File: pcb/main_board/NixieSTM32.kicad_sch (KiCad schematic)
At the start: 36 parts, among them J1 Conn_ARM_SWD_6, Q1 FQU11P06TU, SW1 SW_SPDT, U1 STM32L010K4T6, U2 MAX6817, U3 TPS7A05SOT23, U4 LT3470ITS8PBF, Y1 32.768kHz

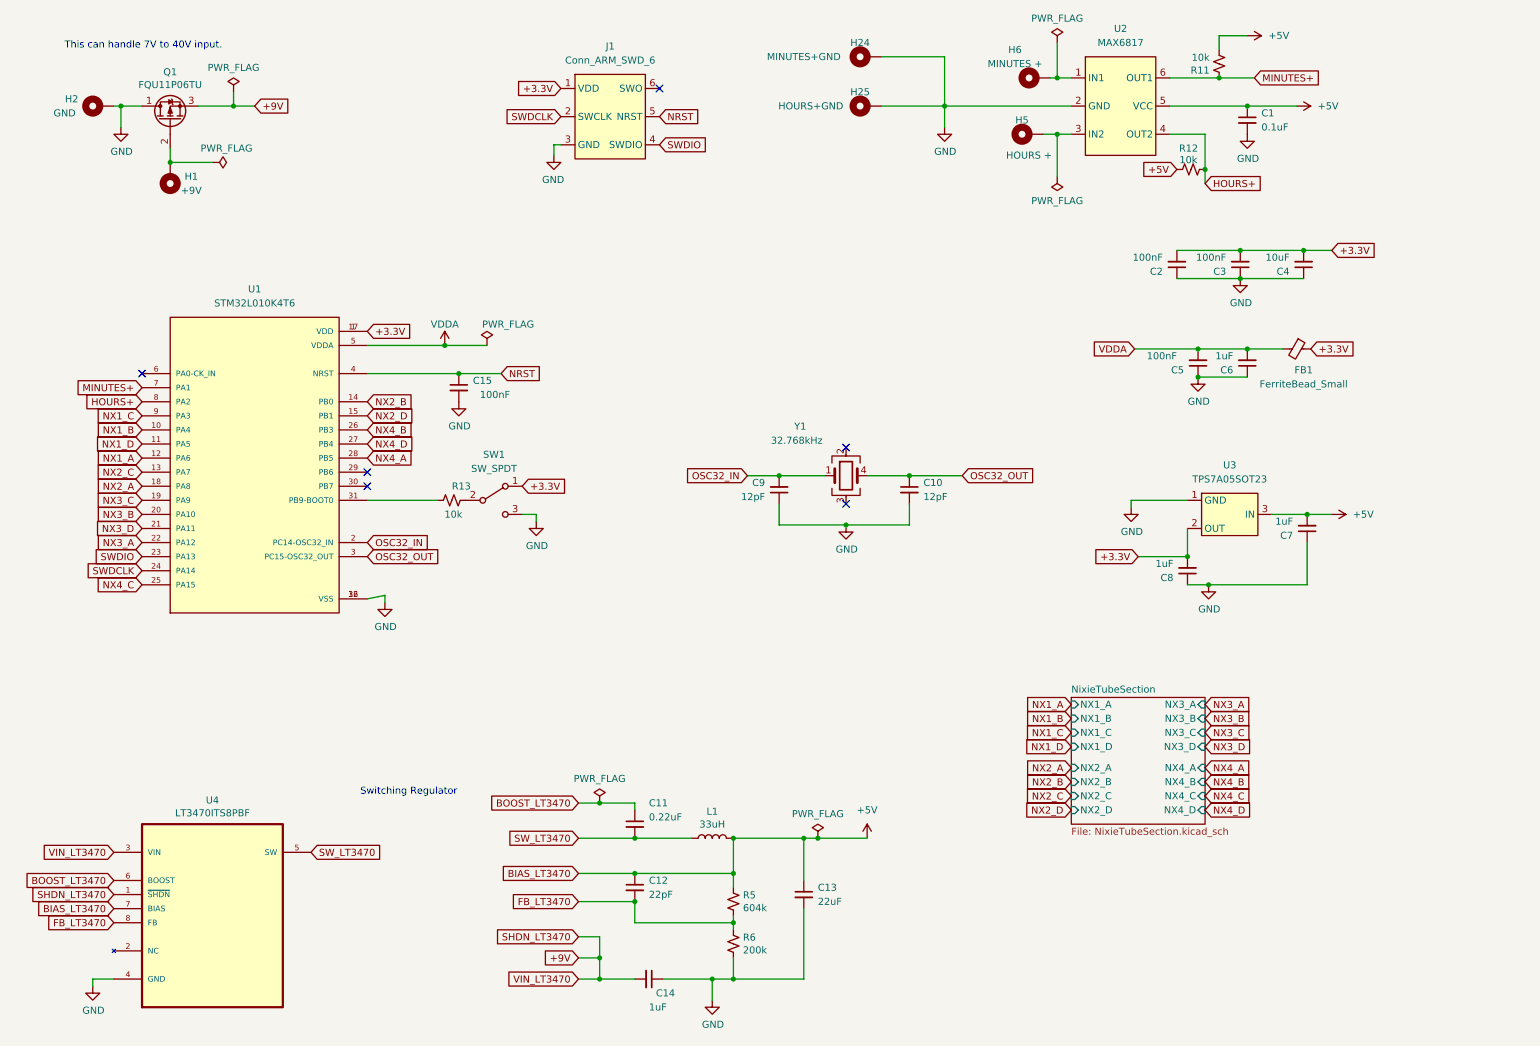
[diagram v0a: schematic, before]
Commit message: Adding images and updating README.
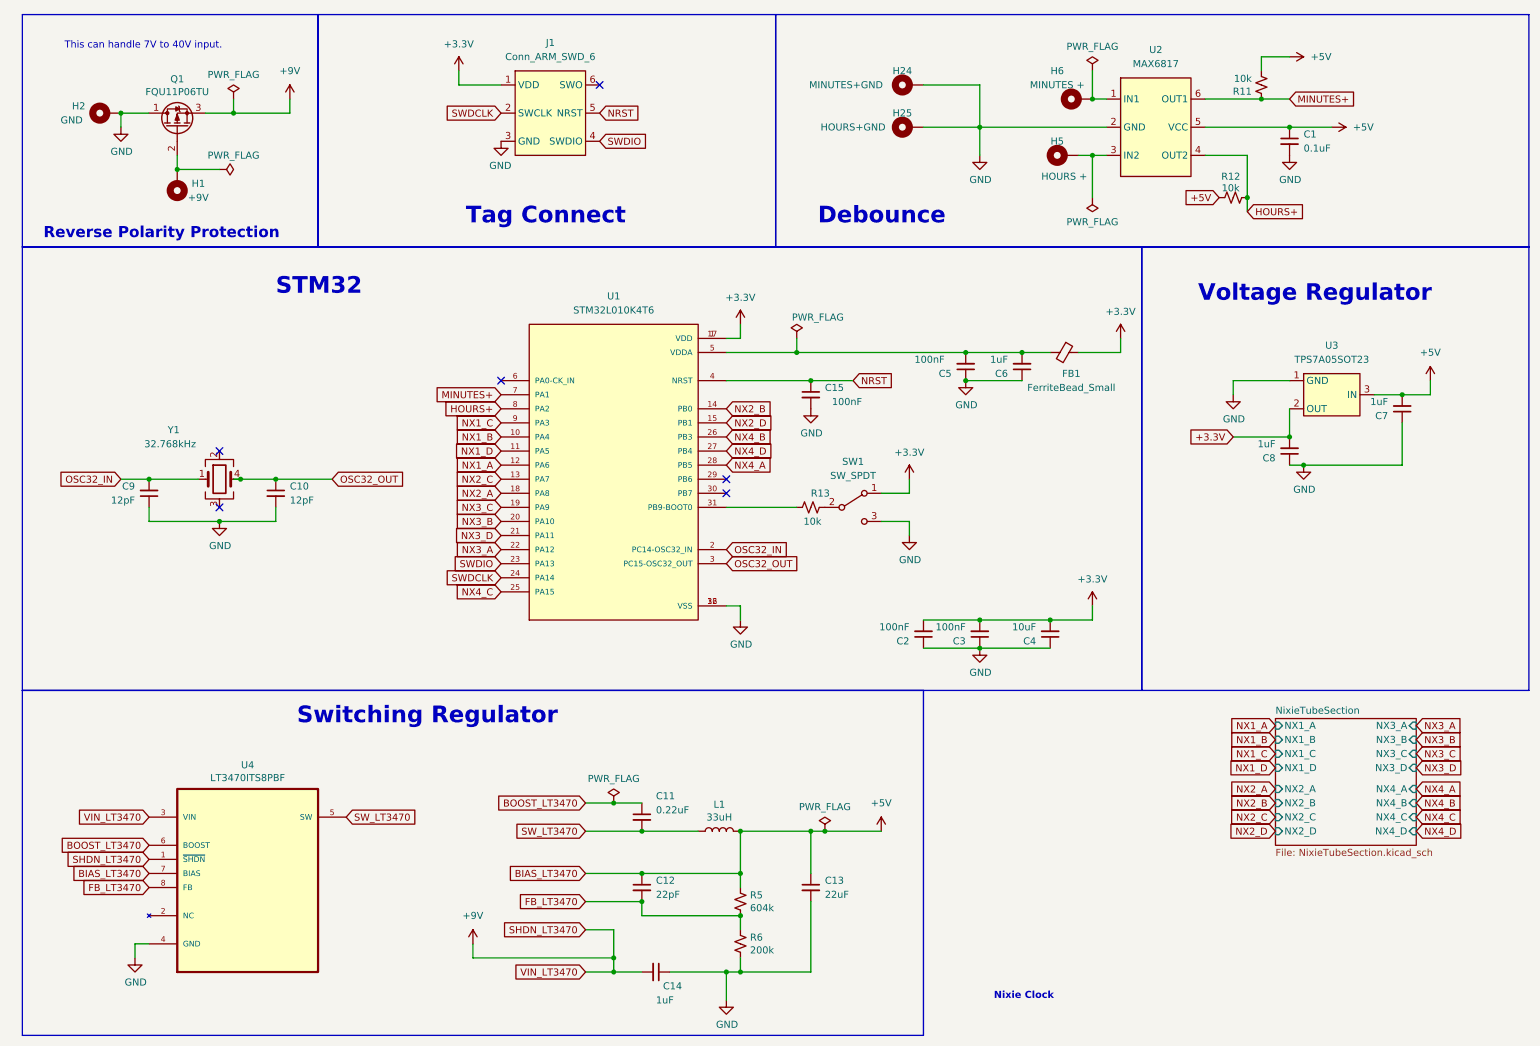
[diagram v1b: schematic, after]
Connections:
- net VDDA: no longer names the net of C5.2, C6.2, FB1.2, U1.5 (VDDA)
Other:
- note added: "Debounce"
- note added: "Nixie Clock"
- note added: "Reverse Polarity Protection"
- note added: "STM32"
- note added: "Tag Connect"
- note added: "Voltage Regulator"
- moved on the sheet: C1, C10, C11, C12, C13, C14, C15, C2, C3, C4, C5, C6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
